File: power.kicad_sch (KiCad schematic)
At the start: 28 parts, among them J3 Conn_01x02_MountingPin, J4 Conn_01x02_Socket, J5 Conn_01x02_Socket, U3 TPS55287, U4 MPM3620A

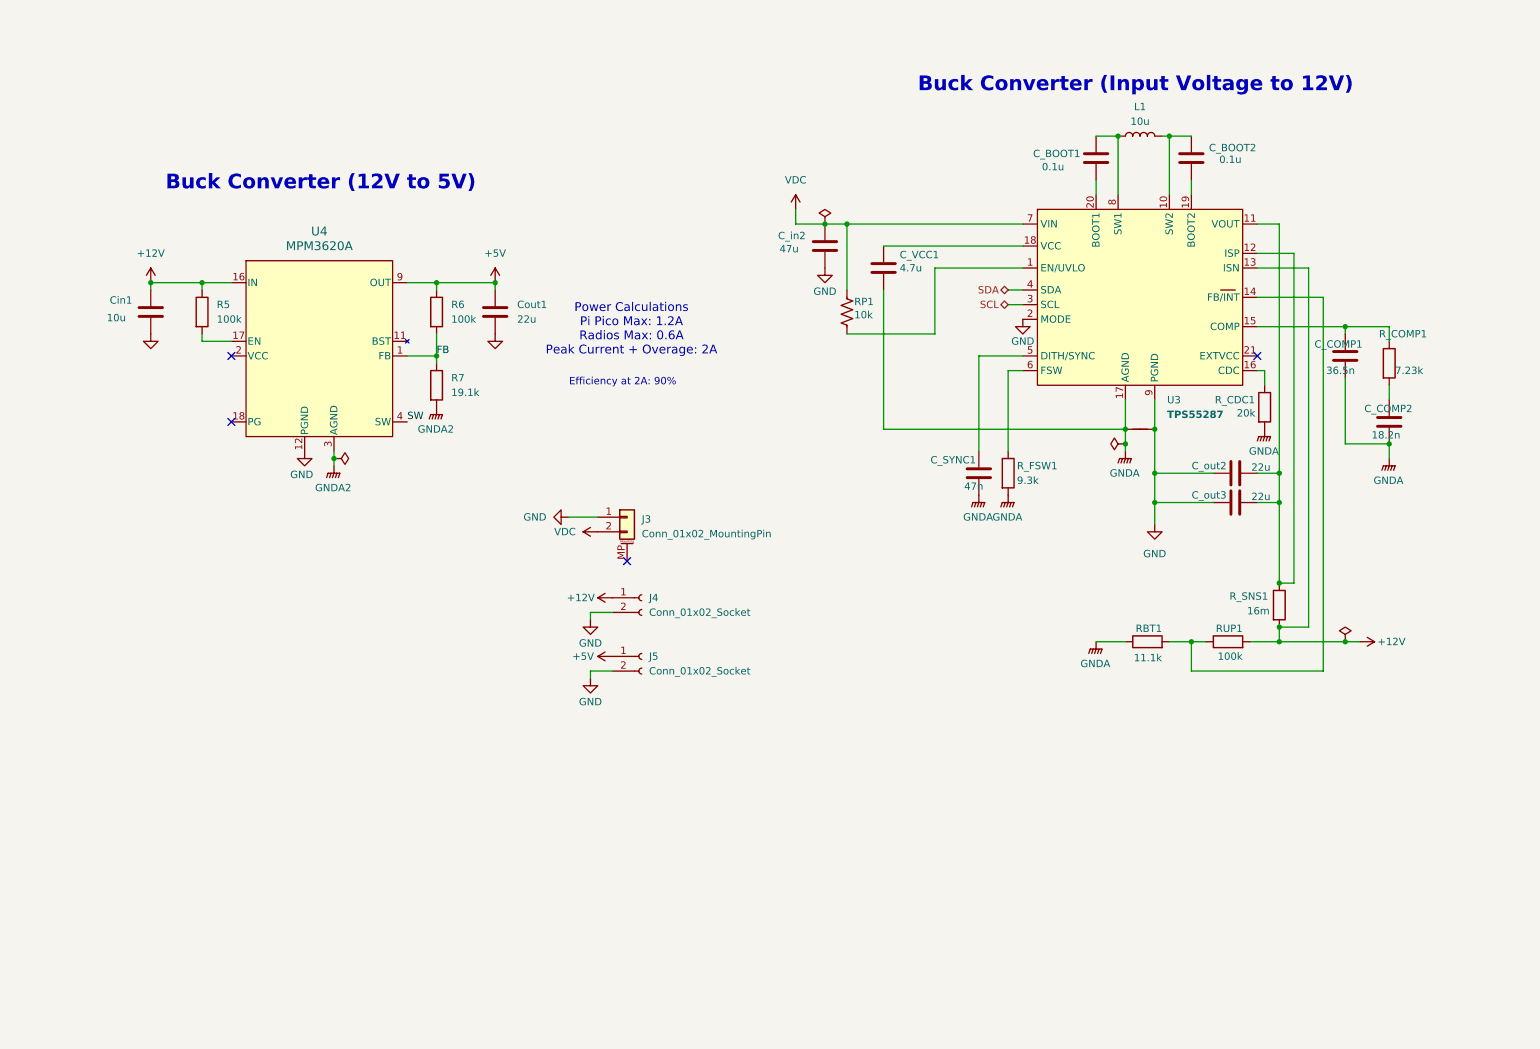
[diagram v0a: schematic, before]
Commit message: Power board complete v1.0
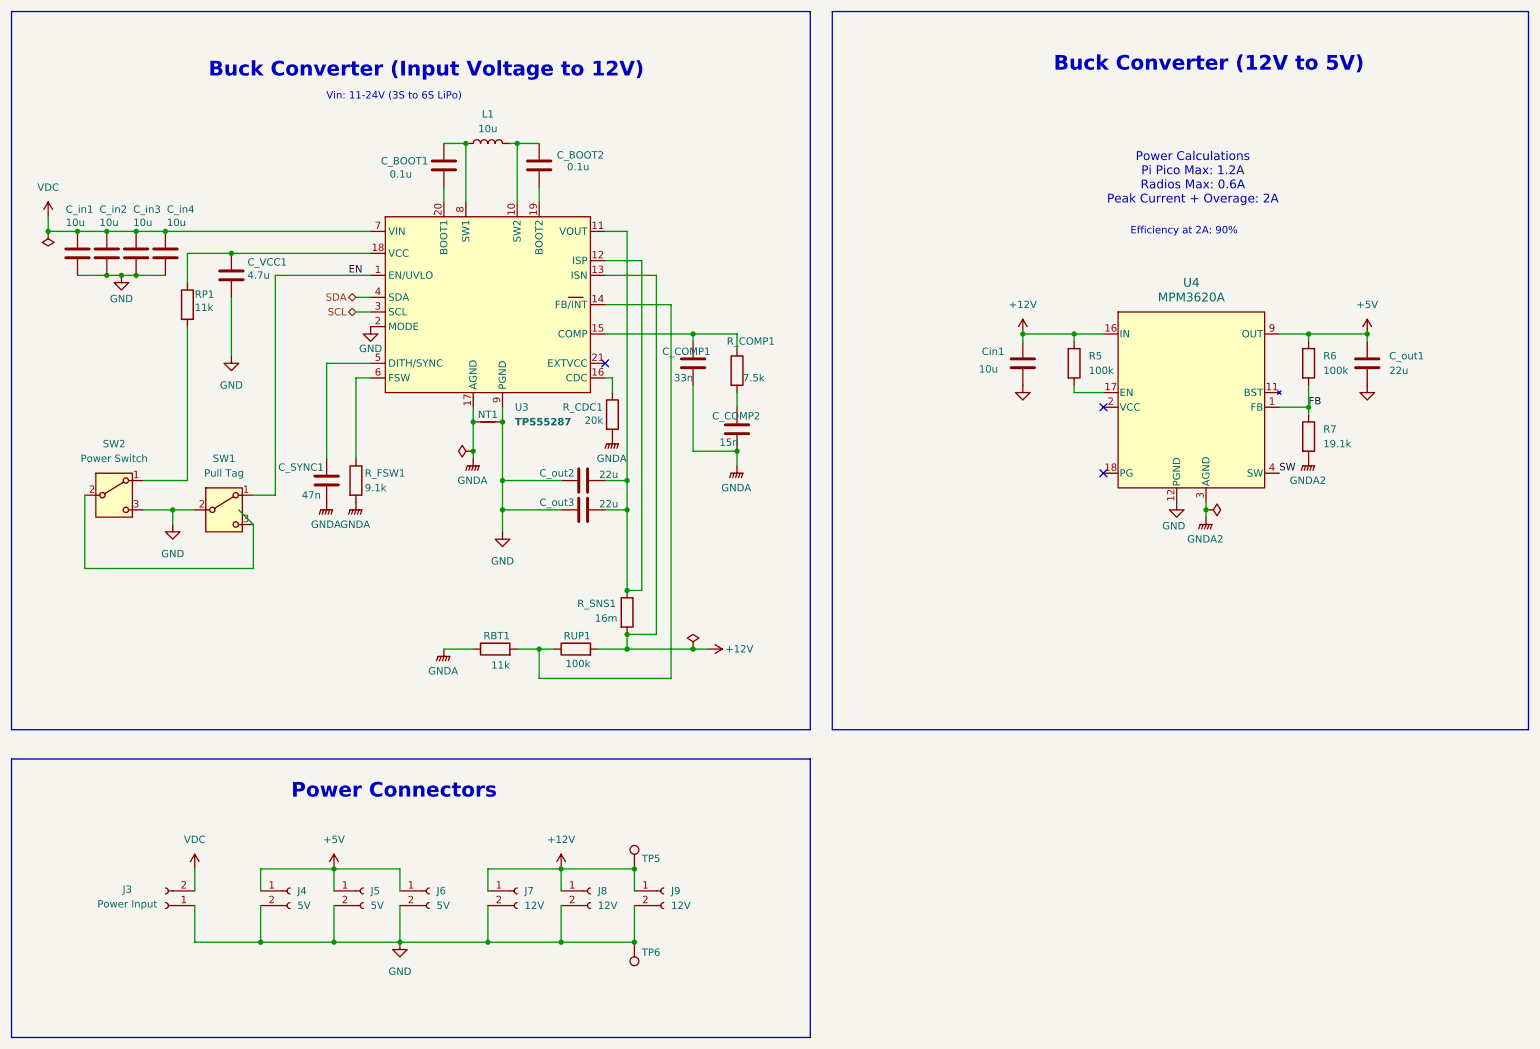
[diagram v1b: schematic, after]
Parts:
- added C_in1, C_in3, C_in4: 10u, Capacitor_SMD:C_1206_3216Metric, symbol Device:C
- added J5, J6: 5V, Connector_JST:JST_XH_S2B-XH-A_1x02_P2.50mm_Horizontal, symbol Connector:Conn_01x02_Socket
- added J8, J9: 12V, Connector_JST:JST_XH_S2B-XH-A_1x02_P2.50mm_Horizontal, symbol Connector:Conn_01x02_Socket
- added SW1: Pull Tag, LEOS:D2F-FL-A1, symbol Switch:SW_SPDT
- added SW2: Power Switch, Button_Switch_THT:SW_Slide_SPDT_Angled_CK_OS102011MA1Q, symbol Switch:SW_SPDT
- added TP5: 12V Test, TestPoint:TestPoint_Loop_D2.60mm_Drill0.9mm_Beaded, symbol Connector:TestPoint
- added TP6: GND Test Point, TestPoint:TestPoint_Loop_D2.60mm_Drill0.9mm_Beaded, symbol Connector:TestPoint
- C_COMP1: value 36.5n -> 33n; footprint Capacitor_SMD:C_0805_2012Metric -> Capacitor_SMD:C_0603_1608Metric; Digikey (none) -> 1276-2040-1-ND; MPN (none) -> CL10B333KB8NFNC; Manufacturer (none) -> Samsung Electro-Mechanics
- C_COMP2: value 18.2n -> 15n; footprint Capacitor_SMD:C_0805_2012Metric -> Capacitor_SMD:C_0603_1608Metric; Digikey (none) -> 1276-1277-1-ND; MPN (none) -> CL10B153KB8NNNC; Manufacturer (none) -> Samsung Electro-Mechanics
- C_SYNC1: footprint Capacitor_SMD:C_0805_2012Metric -> Capacitor_SMD:C_0603_1608Metric; Digikey (none) -> 1276-1063-1-ND; MPN (none) -> CL10B473KB8NNNC; Manufacturer (none) -> Samsung Electro-Mechanics
- C_VCC1: Digikey (none) -> 1276-2970-1-ND; MPN (none) -> CL21B475KOFNFNE; Manufacturer (none) -> Samsung Electro-Mechanics
- C_in2: value 47u -> 10u; footprint Capacitor_SMD:C_0805_2012Metric -> Capacitor_SMD:C_1206_3216Metric; Digikey (none) -> 1276-6767-1-ND; MPN (none) -> CL31B106KBHNNNE; Manufacturer (none) -> Samsung Electro-Mechanics
- J3: value Conn_01x02_MountingPin -> Power Input; footprint Connector_AMASS:AMASS_XT60IPW-M_1x03_P7.20mm_Horizontal -> LEOS:AMASS_XT60IPW-M_1x03_P7.20mm_Horizontal; symbol Connector_Generic_MountingPin:Conn_01x02_MountingPin -> Connector:Conn_01x02_Socket
- J4: renamed from J5; value Conn_01x02_Socket -> 5V; Digikey (none) -> 455-S2B-XH-A-ND; MPN (none) -> S2B-XH-A; Manufacturer (none) -> JST
- J7: renamed from J4; value Conn_01x02_Socket -> 12V; Digikey (none) -> 455-S2B-XH-A-ND; MPN (none) -> S2B-XH-A; Manufacturer (none) -> JST
- L1: Digikey (none) -> 587-2960-1-ND; MPN (none) -> NRS8030T100MJGJ; Manufacturer (none) -> Taiyo Yuden
- NT1: footprint (none) -> NetTie:NetTie-2_SMD_Pad0.5mm
- R5, R6, RUP1: Digikey (none) -> 541-100KCCT-ND; MPN (none) -> CRCW0805100KFKEA; Manufacturer (none) -> Vishay Dale
- R7: Digikey (none) -> 541-19.1KCCT-ND; MPN (none) -> CRCW080519K1FKEA; Manufacturer (none) -> Vishay Dale
- RBT1: value 11.1k -> 11k; Digikey (none) -> 541-CRCW080511K0FKEACCT-ND; MPN (none) -> CRCW080511K0FKEAC; Manufacturer (none) -> Vishay Dale
- RP1: value 10k -> 11k; symbol Device:R_US -> Device:R; Digikey (none) -> 541-CRCW080511K0FKEACCT-ND; MPN (none) -> CRCW080511K0FKEAC; Manufacturer (none) -> Vishay Dale
- R_CDC1: Digikey (none) -> 541-20.0KCCT-ND; MPN (none) -> CRCW080520K0FKEA; Manufacturer (none) -> Vishay Dale
- R_COMP1: value 7.23k -> 7.5k; Digikey (none) -> 541-CRCW08057K50FKEACCT-ND; MPN (none) -> CRCW08057K50FKEAC; Manufacturer (none) -> Vishay Dale
- R_FSW1: value 9.3k -> 9.1k; Digikey (none) -> 541-9.10KCCT-ND; MPN (none) -> CRCW08059K10FKEA; Manufacturer (none) -> Vishay Dale
- R_SNS1: Digikey (none) -> 541-WSLP0805R0160FEACT-ND; MPN (none) -> WSLP0805R0160FEA; Manufacturer (none) -> Vishay Dale
- renumbered Cout1 to C_out1
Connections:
- net +12V: now also J8.1 (Pin_1), J9.1 (Pin_1), TP5.1
- net +5V: now also J5.1 (Pin_1), J6.1 (Pin_1)
- net GND: now also C_VCC1.2, C_in1.2, C_in3.2, C_in4.2, J5.2 (Pin_2), J6.2 (Pin_2), J8.2 (Pin_2), J9.2 (Pin_2), SW1.2 (B), SW2.3 (C), TP6.1
- net GNDA: no longer C_VCC1.2
- net VDC: now also C_in1.1, C_in3.1, C_in4.1; no longer RP1.1
- net at C_VCC1.1, U3.18 (VCC): now also RP1.1
- net at RP1.2: now also SW2.1 (A); no longer U3.1 (EN/UVLO)
- new net: SW1.3 (C), SW2.2 (B)
- new net EN: SW1.1 (A), U3.1 (EN/UVLO)
- no-connect marks 4 -> 3
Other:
- note added: "Power Connectors"
- note added: "Vin: 11-24V (3S to 6S LiPo)"
- moved on the sheet: C_BOOT1, C_BOOT2, C_COMP1, C_COMP2, C_SYNC1, C_VCC1, C_in2, C_out1, C_out2, C_out3, Cin1, J4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
